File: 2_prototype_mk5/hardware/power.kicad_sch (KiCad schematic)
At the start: 34 parts, among them U6 TPS63020DSJR, U8 TPS25921ADR, U9 TPS61094DSSR

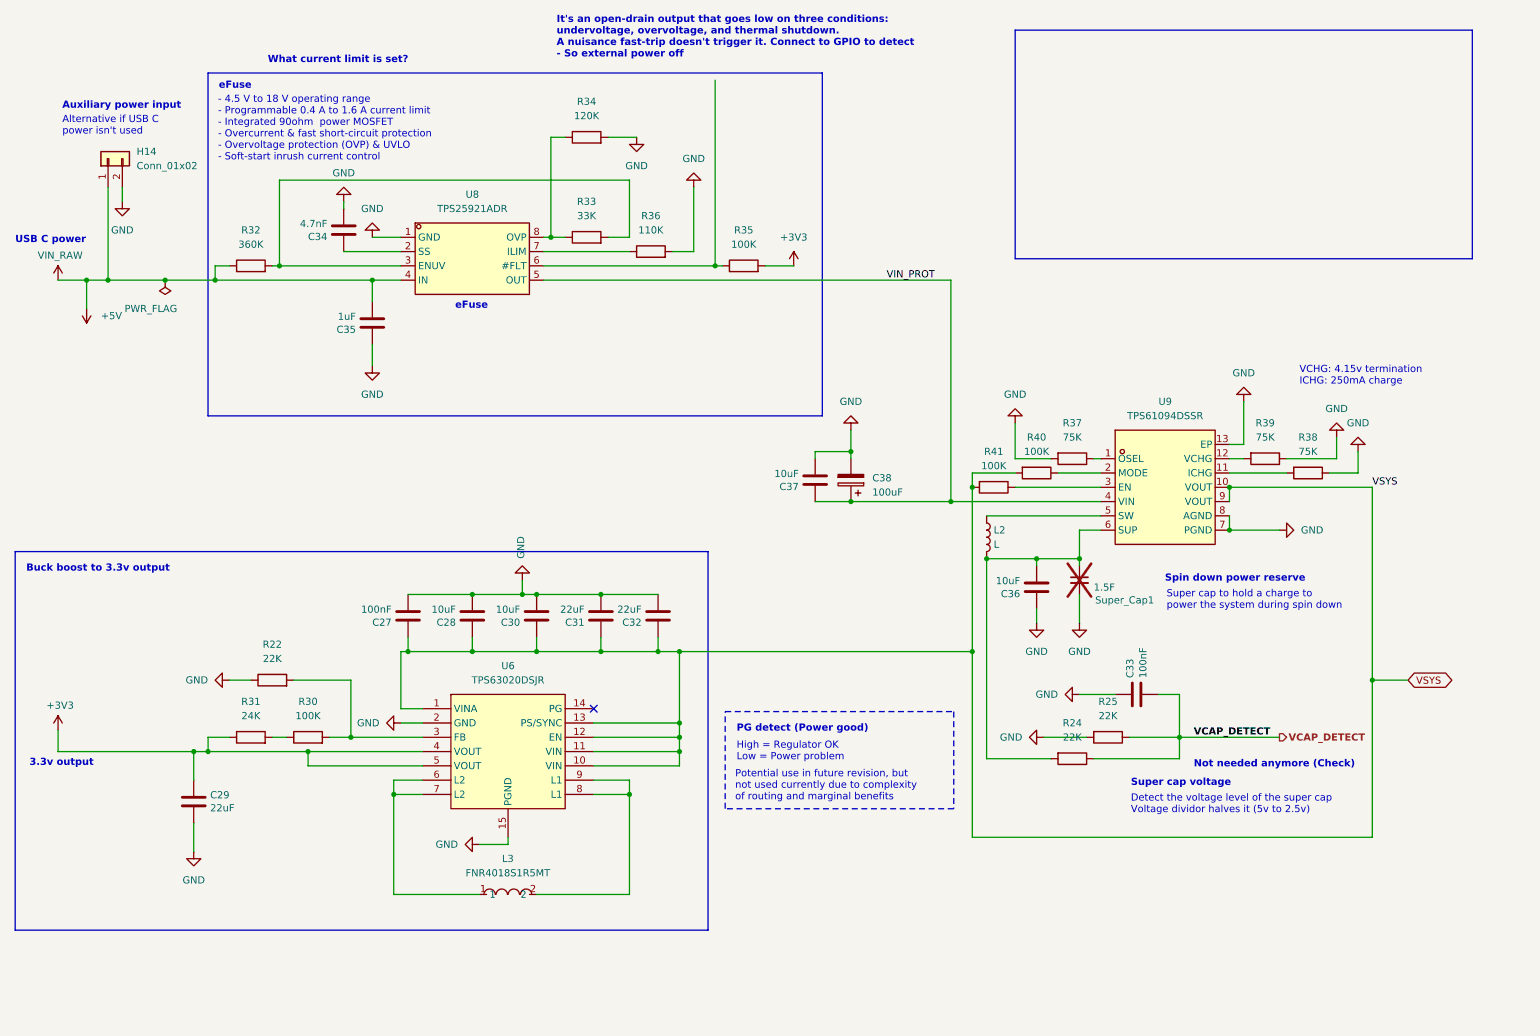
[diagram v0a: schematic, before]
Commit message: Tweaks
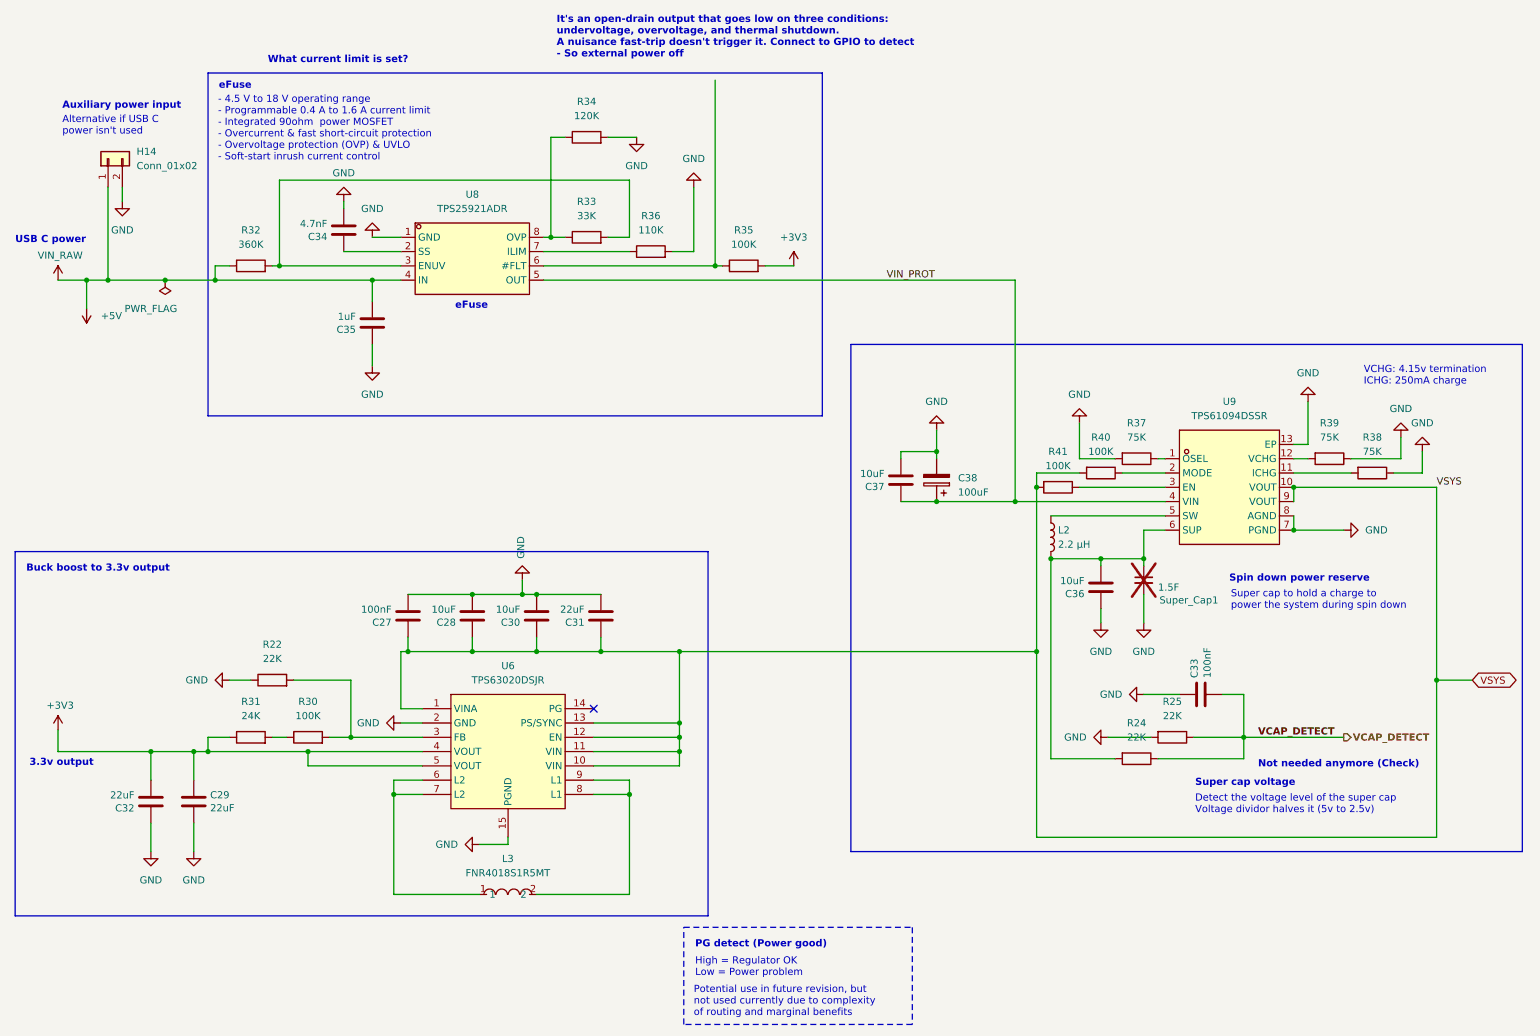
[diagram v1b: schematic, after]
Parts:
- L2: value L -> 2.2 µH; footprint (none) -> easyeda2kicad:IND-SMD_L4.0-W4.0_FNR40XXS
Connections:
- net +3V3: now also C32.2
- net GND: now also C32.1; no longer C32.2
- net VSYS: no longer C32.1
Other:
- moved on the sheet: C33, C36, C37, C38, L2, R24, R25, R37, R38, R39, R40, R41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
